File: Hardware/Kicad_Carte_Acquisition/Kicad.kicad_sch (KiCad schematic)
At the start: 54 parts, among them J1_Vphase1 Conn_01x01, J2_Vphase2 Conn_01x01, J3_Vphase3 Conn_01x01, J4_Neutre1 Conn_01x01, J5_Ph_230V1 Conn_01x01, J6_Neutre_230V1 Conn_01x01, P1 DA15_Receptacle_MountingHoles, U1 LV25-P, U10 OP275, U11 OP275, U12 TMP-15-215, U2 LV25-P, U3 LV25-P, U4 OP275, U5 OP275, U6 OP275, U7 LM2937xS, U8 OP275, U9 OP275

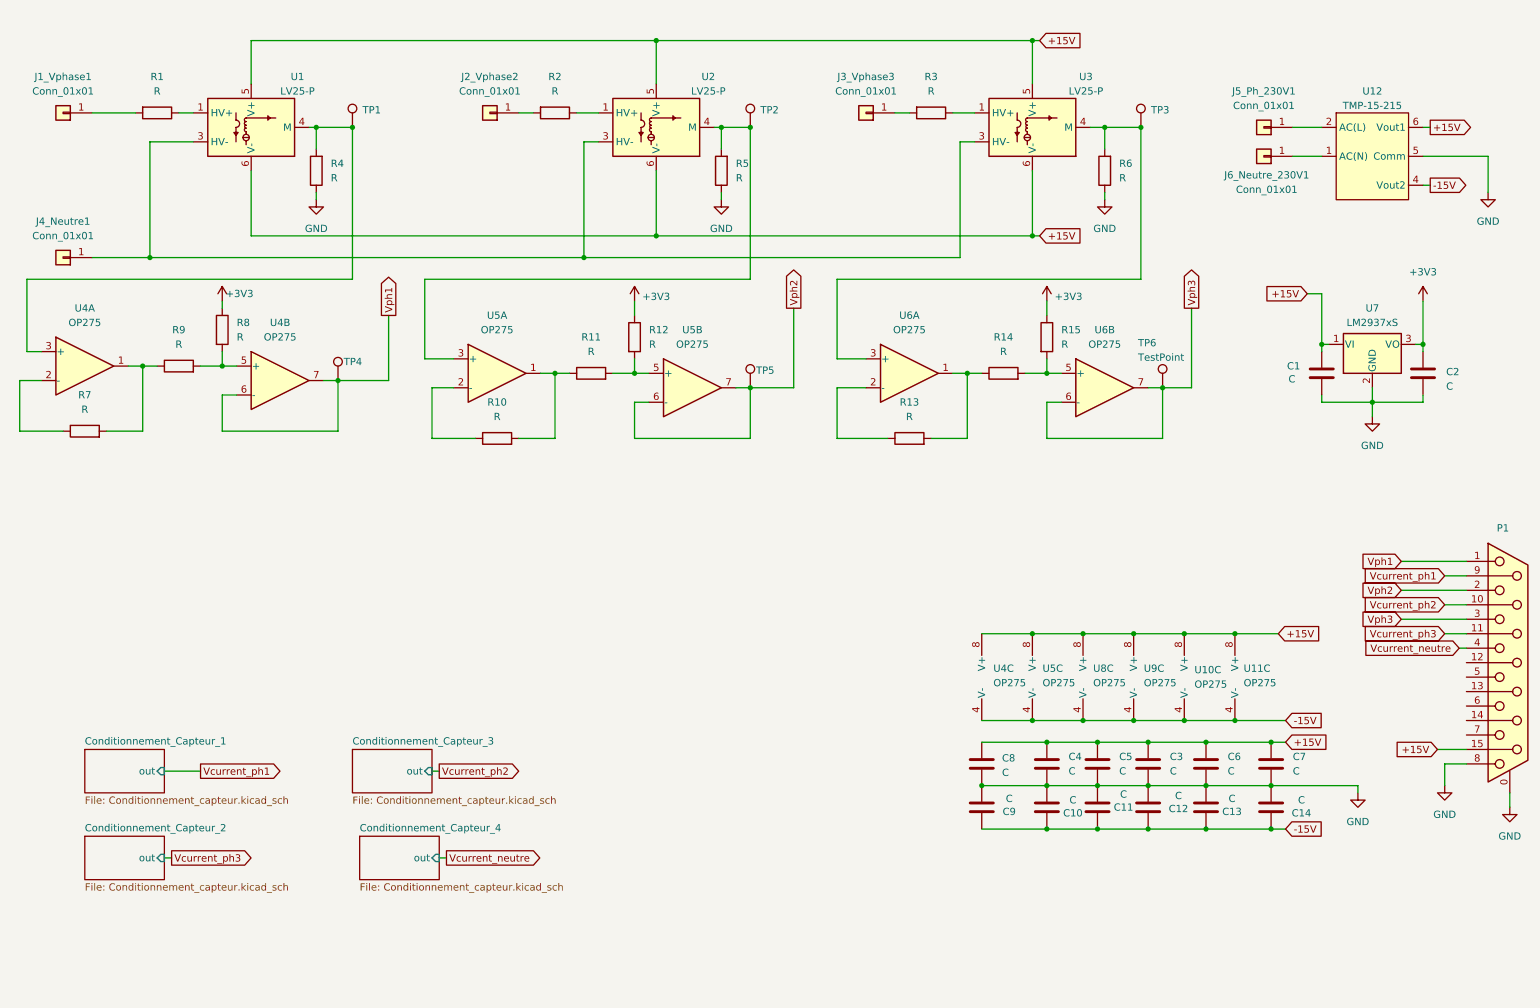
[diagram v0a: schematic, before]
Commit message: modif
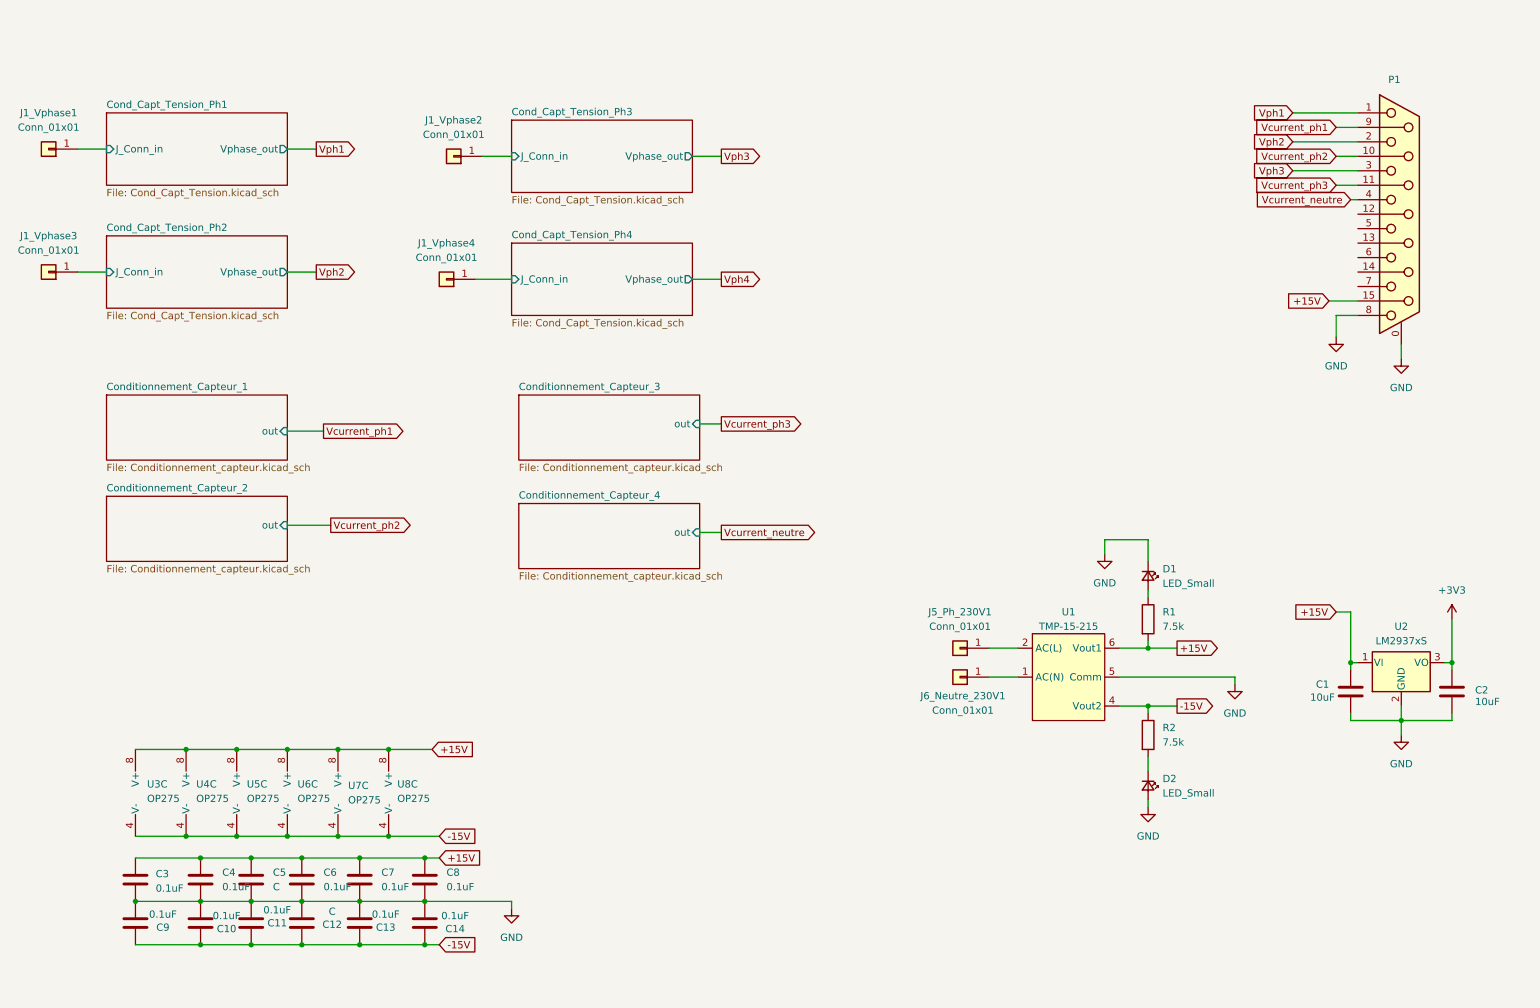
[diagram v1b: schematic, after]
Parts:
- removed J2_Vphase2, J3_Vphase3, J4_Neutre1: Conn_01x01, Connector:Banana_Cliff_FCR7350B_S16N-PC_Horizontal, symbol Connector_Generic:Conn_01x01
- removed R10, R11, R12, R13, R14, R15, R3, R4, R5, R6, R7, R8, R9: R, symbol Device:R
- removed TP1, TP2, TP3, TP4, TP5, TP6: TestPoint, symbol Connector:TestPoint
- removed U1, U2, U3: LV25-P, Sensor_Voltage:LEM_LV25-P, symbol Sensor_Voltage:LV25-P
- removed unit 2 of U4
- removed unit 1 of U4
- removed unit 1 of U5
- removed unit 2 of U5
- removed U6: OP275, symbol Amplifier_Operational:OP275
- added D1, D2: LED_Small, symbol Device:LED_Small
- added J1_Vphase2, J1_Vphase3, J1_Vphase4: Conn_01x01, Connector:Banana_Cliff_FCR7350B_S16N-PC_Horizontal, symbol Connector_Generic:Conn_01x01
- C1, C2: value C -> 10uF
- C10, C11, C13, C14, C4, C9: value C -> 0.1uF
- C3: renamed from C8; value C -> 0.1uF
- C6: renamed from C3; value C -> 0.1uF
- C7: renamed from C6; value C -> 0.1uF
- C8: renamed from C7; value C -> 0.1uF
- R1, R2: value R -> 7.5k
- renumbered U12 to U1, U7 to U2, U4 to U3, U5 to U4, U8 to U5, U9 to U6, U10 to U7, U11 to U8
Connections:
- net +15V: now also R1.2
- net -15V: now also R2.1
- net GND: now also D1.1 (K), D2.2 (A)
- net at R1.1: now also D1.2 (A)
- net Cond_Capt_Tension_Ph1/J_Conn_in: now reaches J1_Vphase1.1 (Pin_1)
- net Cond_Capt_Tension_Ph1/J_Conn_in: no longer R1.2
- net at R2.2: now also D2.1 (K)
- new net Cond_Capt_Tension_Ph2/J_Conn_in: J1_Vphase3.1 (Pin_1)
- new net Cond_Capt_Tension_Ph3/J_Conn_in: J1_Vphase2.1 (Pin_1)
- new net Cond_Capt_Tension_Ph4/J_Conn_in: J1_Vphase4.1 (Pin_1)
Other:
- added sheet Cond_Capt_Tension_Ph1 (Cond_Capt_Tension.kicad_sch)
- added sheet Cond_Capt_Tension_Ph2 (Cond_Capt_Tension.kicad_sch)
- added sheet Cond_Capt_Tension_Ph3 (Cond_Capt_Tension.kicad_sch)
- added sheet Cond_Capt_Tension_Ph4 (Cond_Capt_Tension.kicad_sch)
- moved on the sheet: C1, C10, C11, C12, C13, C14, C2, C3, C4, C5, C6, C7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

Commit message: modif
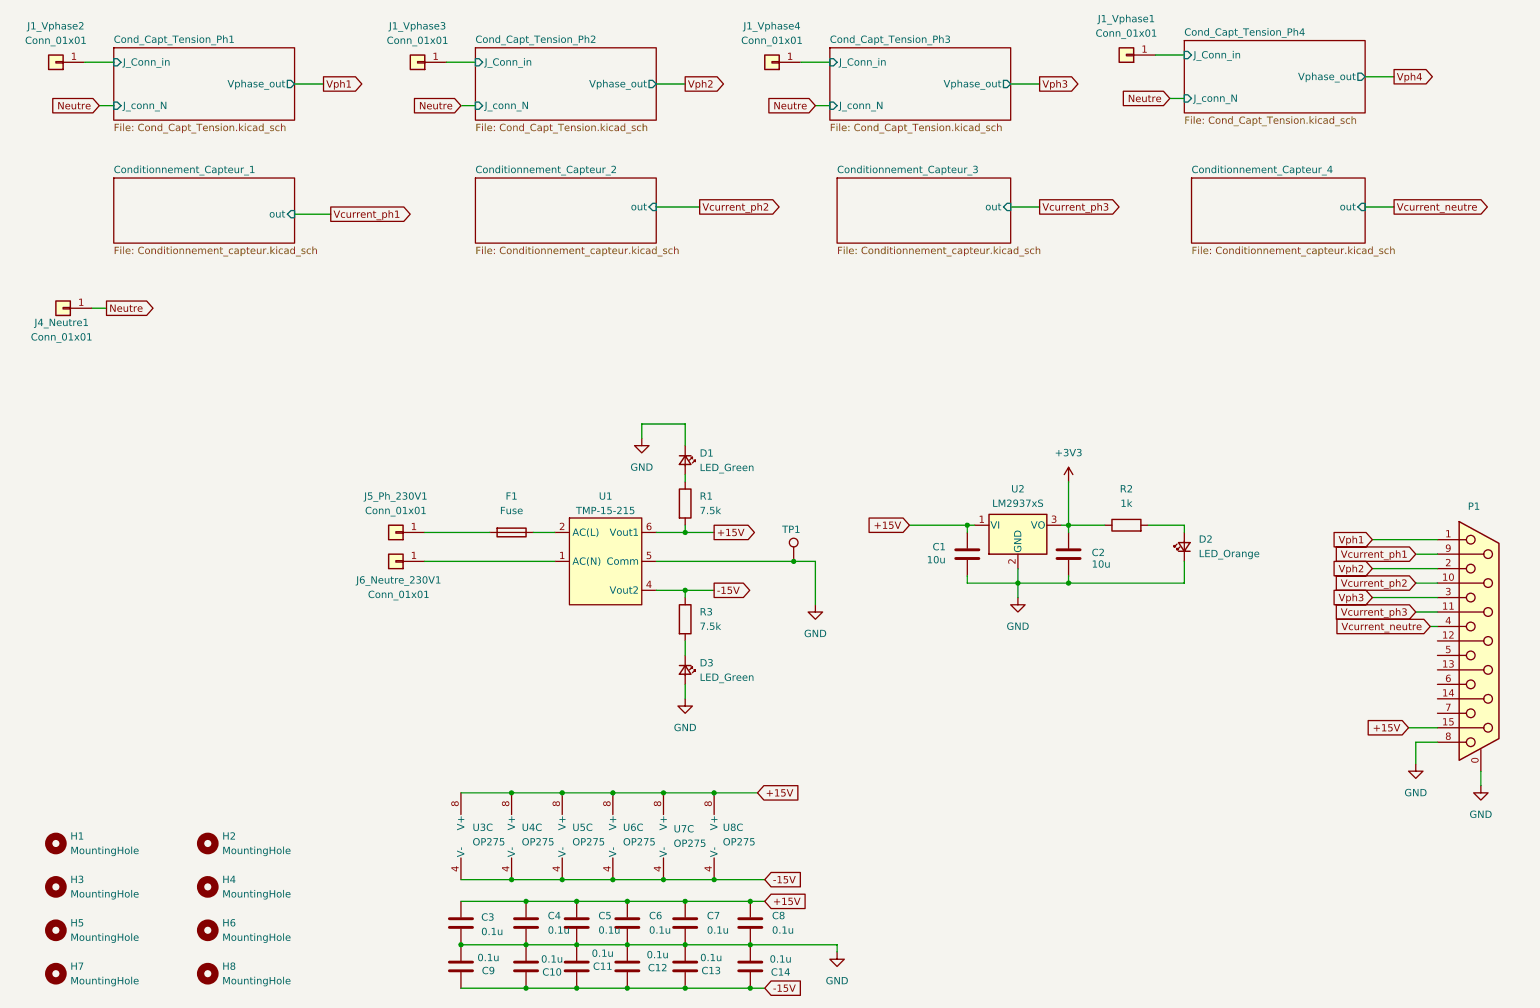
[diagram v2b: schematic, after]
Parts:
- added D2: LED_Orange, LED_SMD:LED_0603_1608Metric_Pad1.05x0.95mm_HandSolder, symbol Device:LED_Small
- added F1: Fuse, symbol Device:Fuse
- added H1, H2, H3, H4, H5, H6, H7, H8: MountingHole, symbol Mechanical:MountingHole
- added J4_Neutre1: Conn_01x01, Connector:Banana_Cliff_FCR7350B_S16N-PC_Horizontal, symbol Connector_Generic:Conn_01x01
- added R2: 1k, Resistor_SMD:R_0805_2012Metric_Pad1.20x1.40mm_HandSolder, symbol Device:R
- added TP1: TestPoint, symbol Connector:TestPoint
- C1, C2: value 10uF -> 10u; footprint (none) -> Capacitor_SMD:C_0805_2012Metric_Pad1.18x1.45mm_HandSolder
- C10, C11, C13, C14, C3, C4, C6, C7, C8, C9: value 0.1uF -> 0.1u; footprint (none) -> Capacitor_SMD:C_0805_2012Metric_Pad1.18x1.45mm_HandSolder
- C12, C5: value C -> 0.1u; footprint (none) -> Capacitor_SMD:C_0805_2012Metric_Pad1.18x1.45mm_HandSolder
- D1: value LED_Small -> LED_Green; footprint (none) -> LED_SMD:LED_0603_1608Metric_Pad1.05x0.95mm_HandSolder
- D3: renamed from D2; value LED_Small -> LED_Green; footprint (none) -> LED_SMD:LED_0603_1608Metric_Pad1.05x0.95mm_HandSolder
- R1: footprint (none) -> Resistor_SMD:R_0805_2012Metric_Pad1.20x1.40mm_HandSolder
- R3: renamed from R2; footprint (none) -> Resistor_SMD:R_0805_2012Metric_Pad1.20x1.40mm_HandSolder
- U3, U4, U5, U6, U7, U8: footprint (none) -> Package_SO:SOIC-8_3.9x4.9mm_P1.27mm
- renumbered J1_Vphase4 to J1_Vphase1, J1_Vphase1 to J1_Vphase2, J1_Vphase2 to J1_Vphase4
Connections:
- net +3V3: now also R2.1
- net GND: now also D2.1 (K), TP1.1
- net at U1.2 (AC(L)): now also F1.1; no longer J5_Ph_230V1.1 (Pin_1)
- new net: F1.2, J5_Ph_230V1.1 (Pin_1)
- new net: D2.2 (A), R2.2
- new net Neutre: J4_Neutre1.1 (Pin_1)
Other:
- sheet Cond_Capt_Tension_Ph1 ports: added J_conn_N; removed none
- sheet Cond_Capt_Tension_Ph2 ports: added J_conn_N; removed none
- sheet Cond_Capt_Tension_Ph3 ports: added J_conn_N; removed none
- sheet Cond_Capt_Tension_Ph4 ports: added J_conn_N; removed none
- moved on the sheet: C1, C10, C11, C12, C13, C14, C2, C3, C4, C5, C6, C7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
